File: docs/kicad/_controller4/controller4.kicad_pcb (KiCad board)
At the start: 2 copper layers, 74.9 x 99.1 mm, 32 parts, among them J1 24V, J10 Display, J11 PWM, J2 Z_AXIS, J3 A_AXIS, J4 Y_AXIS, J5 X_AXIS, J6 Conn_01x04, J7 Conn_01x05, J8 USB 5V, J9 WS2812B Strip, M1 BUCK01, M2 SD_TYP0, U1 ESP32_DEV_0

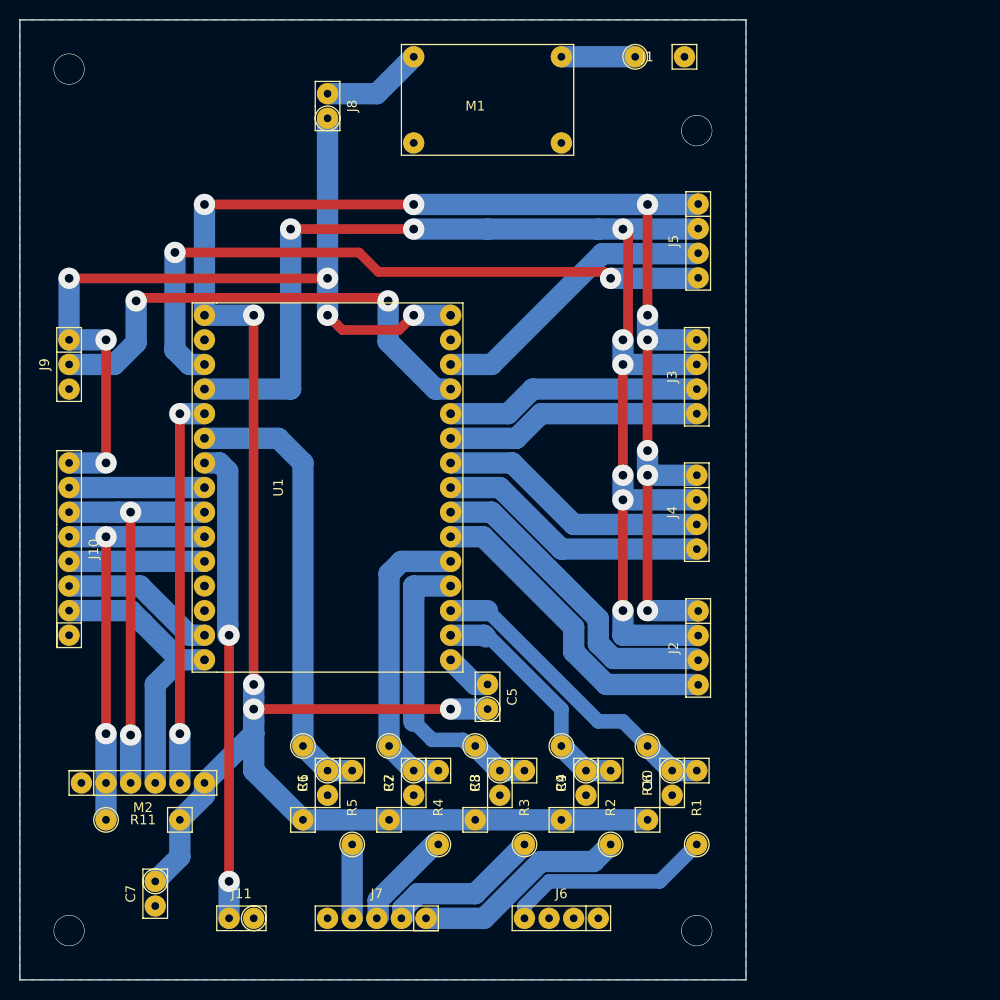
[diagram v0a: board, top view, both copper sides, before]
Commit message: docs - start writing actual documentation
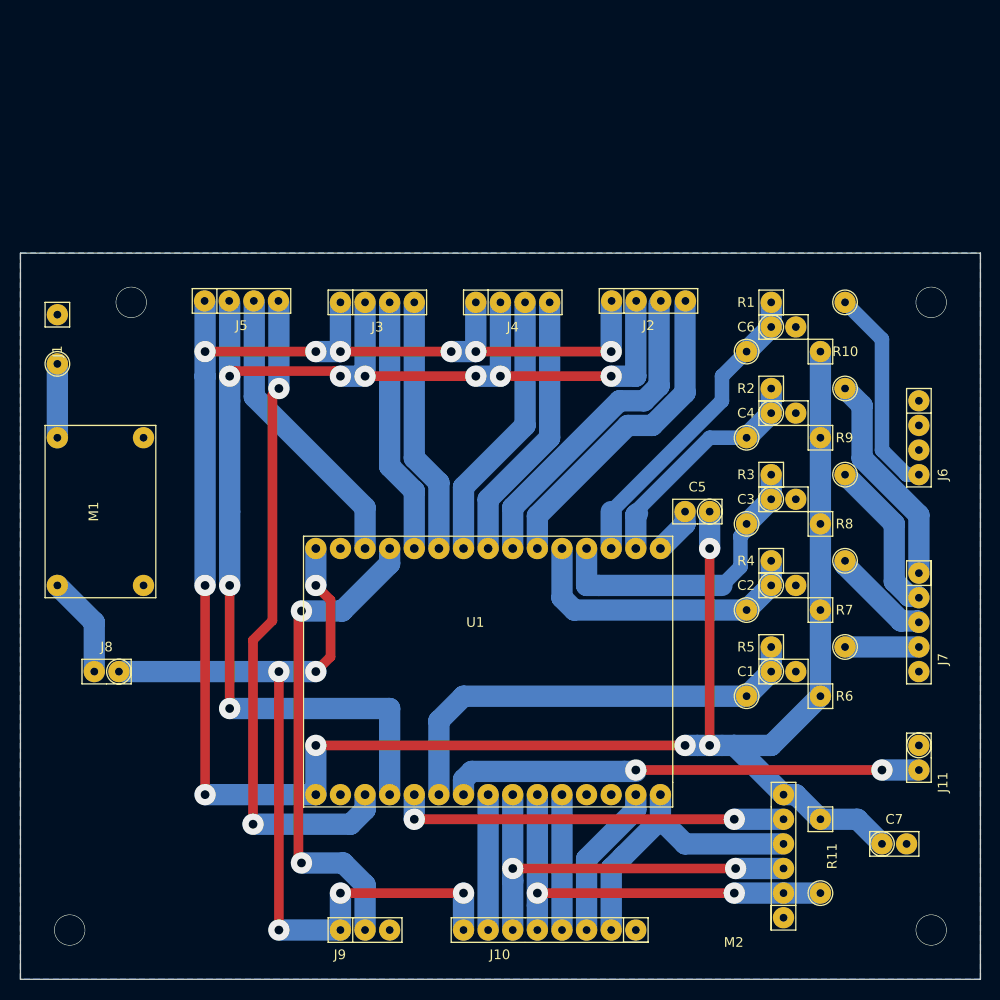
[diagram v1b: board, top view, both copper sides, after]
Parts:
- J10: value Display -> DISPLAY
- J6: value Conn_01x04 -> PROBE
- J7: value Conn_01x05 -> LIMITS
- J9: value WS2812B Strip -> LEDS
- M2: value SD_TYP0 -> SD CARD
- moved C7 75.1 mm to (89.0, -14.0), turned to 0 degrees
- moved M2 73.8 mm to (78.8, -6.35), turned to 90 degrees
- moved J11 70.9 mm to (92.8, -24.1), turned to 270 degrees
- moved J1 70.0 mm to (3.87, -68.6), turned to 270 degrees
- moved R11 66.1 mm to (82.6, -16.5), turned to 270 degrees
- moved J9 65.9 mm to (35.6, -5.08), turned to 0 degrees
- moved J7 63.7 mm to (92.8, -36.8), turned to 270 degrees
- moved J10 63.5 mm to (55.9, -5.08), turned to 180 degrees
- moved J6 62.8 mm to (92.8, -59.7), turned to 270 degrees
- moved J8 61.0 mm to (10.2, -31.8), turned to 180 degrees
- moved R6 54.9 mm to (82.6, -29.2), turned to 180 degrees
- moved M1 52.0 mm to (12.8, -50.8), turned to 270 degrees
- moved J5 51.9 mm to (19.1, -70.0), turned to 0 degrees
- moved R10 51.5 mm to (82.6, -64.8), turned to 180 degrees
- moved R7 49.5 mm to (82.6, -38.1), turned to 180 degrees
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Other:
- board size 74.9 x 99.1 mm -> 99.1 x 74.9 mm
